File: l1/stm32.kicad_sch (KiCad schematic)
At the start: 9 parts, among them J4 Conn_01x04, SW1 SW_Push, Y1 32KHz768

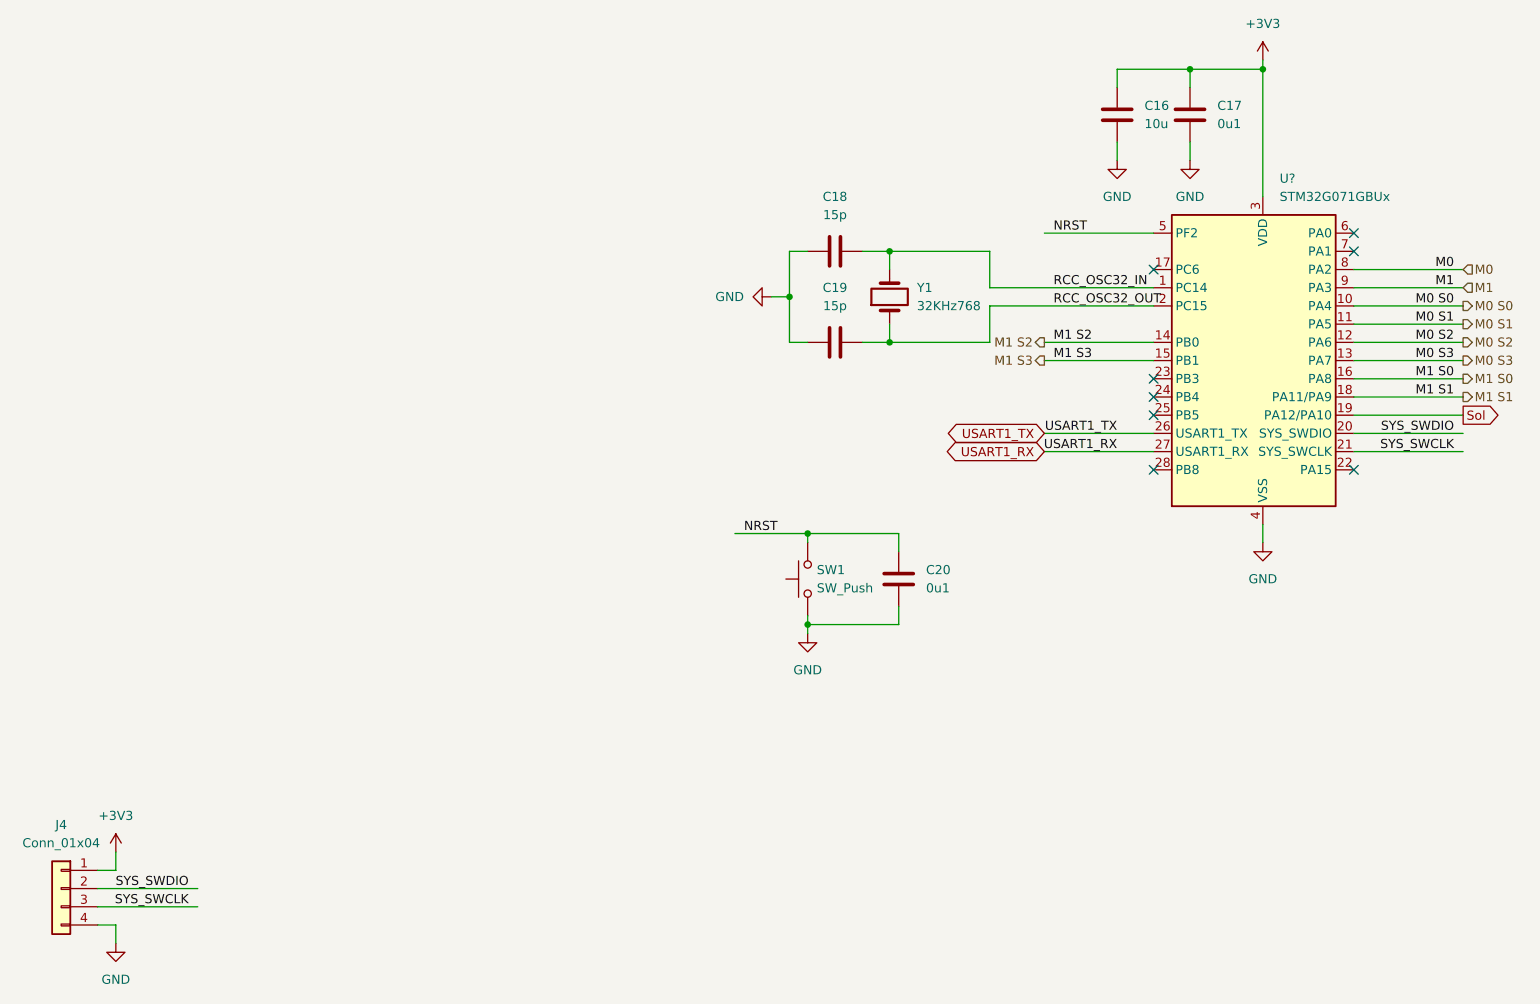
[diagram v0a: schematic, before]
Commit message: Changed To OKL
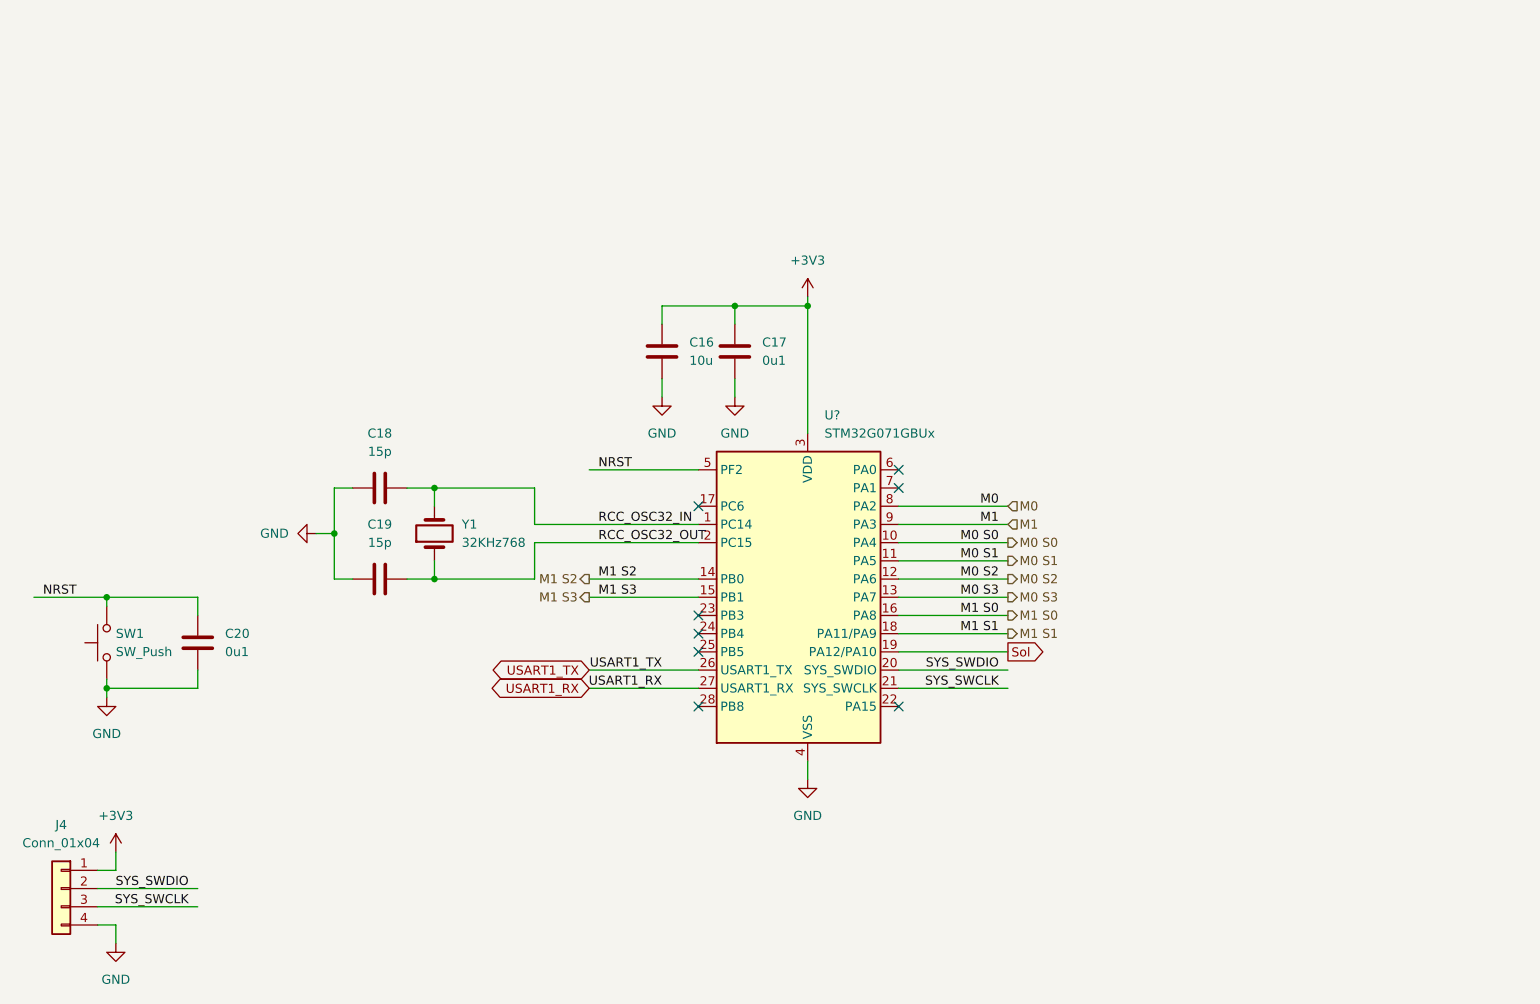
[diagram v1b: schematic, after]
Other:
- moved on the sheet: C16, C17, C18, C19, C20, SW1, U?, Y1
